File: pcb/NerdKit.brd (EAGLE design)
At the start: 148.3 x 69.8 mm, 32 parts, among them U2 ARDUINOR3-PINSONLY

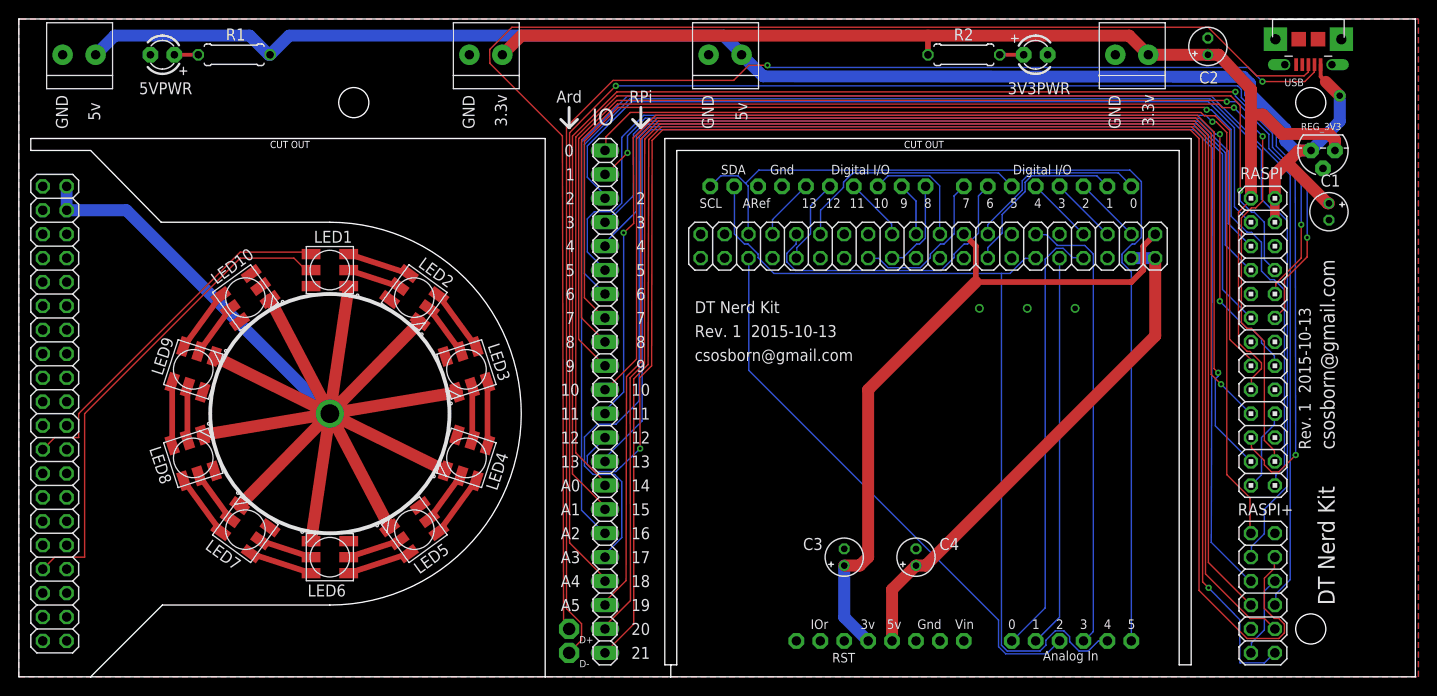
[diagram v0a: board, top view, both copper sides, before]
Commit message: Lots of trace cleanup and local optimizations.
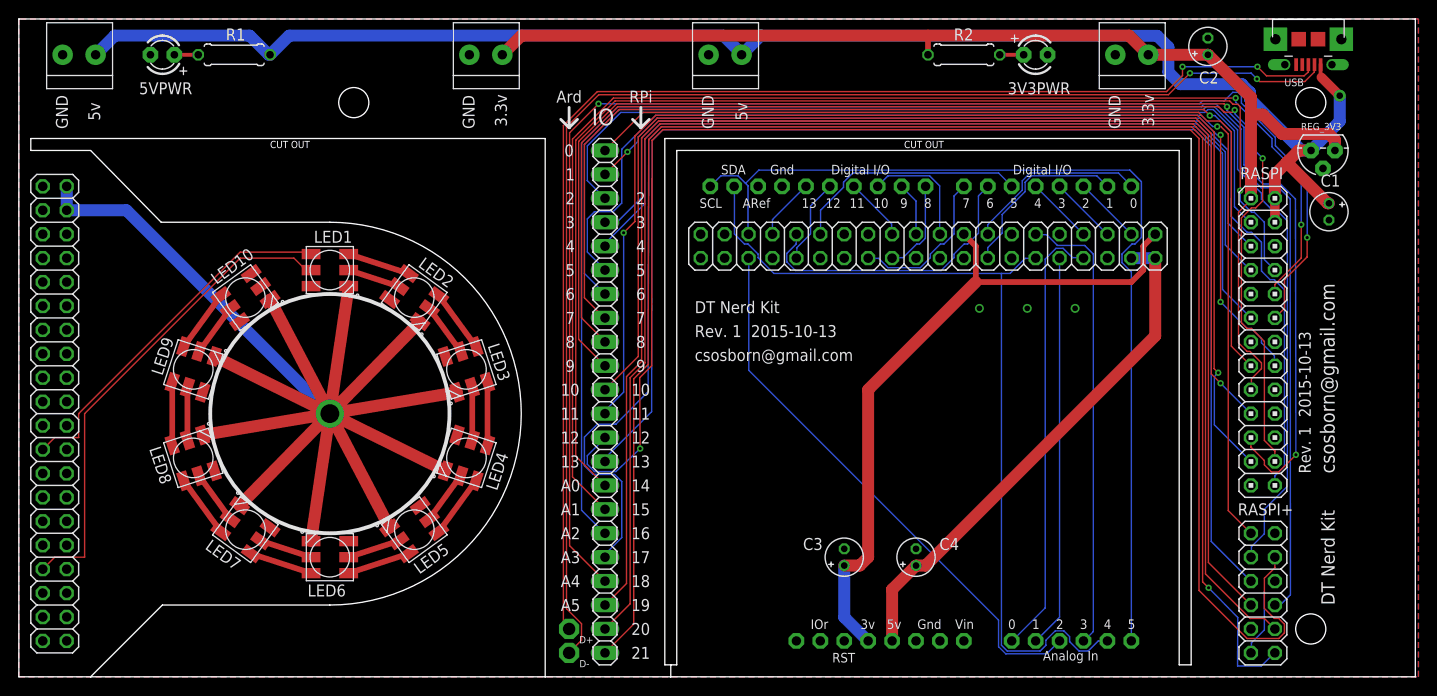
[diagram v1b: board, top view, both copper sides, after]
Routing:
- net N$2: track 156.6 -> 137.9 mm, vias 0 -> 2
- net GND: track 17.4 -> 7.22 mm
- net 5V: track 165.5 -> 167.8 mm
- net GPIO15: track 139.0 -> 137.8 mm
- net GPIO18: track 151.3 -> 150.3 mm
- net GPIO22: track 95.6 -> 94.7 mm
- net GPIO02: track 89.0 -> 88.1 mm
- net GPIO13: track 145.5 -> 144.7 mm
- net GPIO23: track 96.8 -> 96.0 mm
- net GPIO05: track 127.1 -> 126.4 mm
- net GPIO17: track 134.1 -> 133.4 mm
- net GPIO06: track 139.1 -> 138.4 mm
- net GPIO14: track 130.2 -> 129.5 mm
- net GPIO04: track 91.1 -> 90.4 mm
- net N$21: track 141.1 -> 140.4 mm
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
